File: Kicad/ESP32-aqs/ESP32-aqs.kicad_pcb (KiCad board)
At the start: 2 copper layers, 98 x 53.3 mm, 30 parts, among them J1 UART Connector, J2 JST connector SEN55, J3 ufl connector, SW1 RESET, SW2 BOOT, U1 LD1117S33TR_SOT223, U2 ESP32-WROOM-32-N8, U3 SGP41-D-R4, U4 DL-RFM95-868M

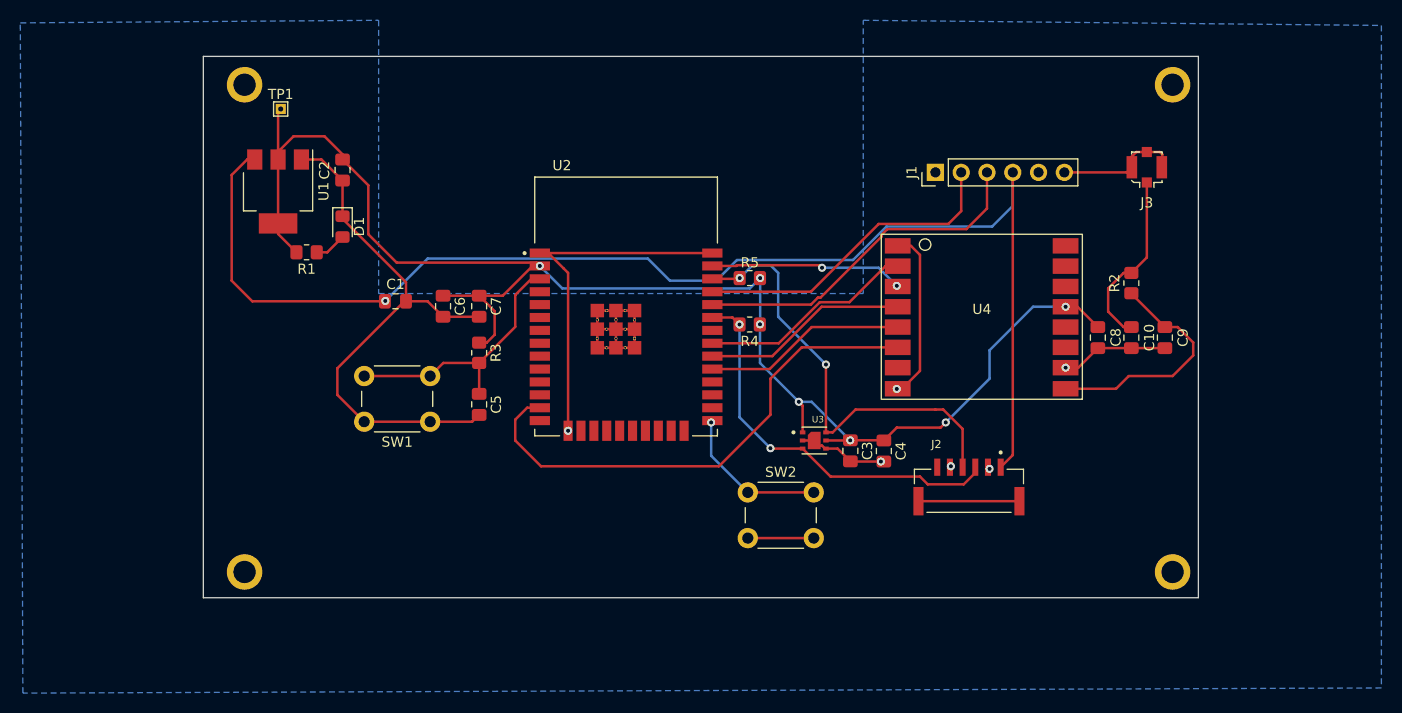
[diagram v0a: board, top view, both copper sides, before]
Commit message: PCB design geupdate
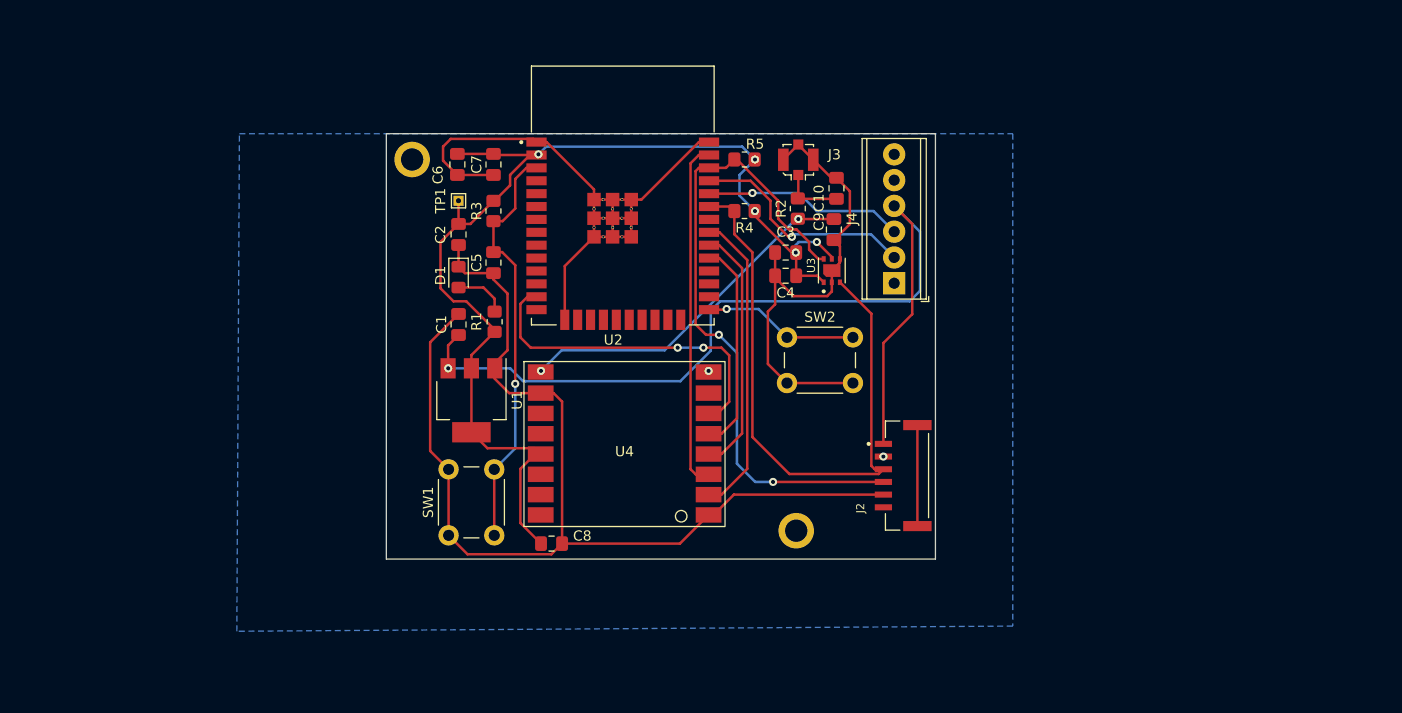
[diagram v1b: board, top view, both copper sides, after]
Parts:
- removed H1, H3: MountingHole, MountingHole:MountingHole_2.2mm_M2_ISO7380_Pad
- removed J1: UART Connector, Connector_PinHeader_2.54mm:PinHeader_1x06_P2.54mm_Vertical
- added J4: UART Connector, TerminalBlock_Phoenix:TerminalBlock_Phoenix_MPT-0,5-6-2.54_1x06_P2.54mm_Horizontal, F.Cu at (183.4, 80.8)
- SW1: value RESET -> TC-1102-B-C-B; footprint Button_Switch_THT:SW_PUSH_6mm_H7.3mm -> Button_Switch_THT:SW_PUSH_6mm
- SW2: value BOOT -> TC-1102-B-C-B; footprint Button_Switch_THT:SW_PUSH_6mm_H7.3mm -> Button_Switch_THT:SW_PUSH_6mm
- U2: value ESP32-WROOM-32-N8 -> ESP32-WROOM-32
- U4: value DL-RFM95-868M -> SX1276S8S+T-X1
- moved C8 57.5 mm to (149.6, 106.4), turned to 0 degrees
- moved H2 37.3 mm to (173.7, 105.2)
- moved U4 37.2 mm to (156.6, 95.6), turned to 0 degrees
- moved J3 34.3 mm to (173.9, 68.6)
- moved C9 34.3 mm to (177.4, 75.5)
- moved R2 33.7 mm to (173.9, 73.4)
- moved C10 32.6 mm to (177.7, 71.4), turned to -90 degrees
- moved U1 28.0 mm to (141.7, 92.3)
- moved C3 20.5 mm to (172.7, 77.7), turned to 180 degrees
- moved C4 19.8 mm to (172.7, 80.0), turned to 180 degrees
- moved R1 19.7 mm to (144.0, 84.6), turned to -90 degrees
- moved TP1 19.7 mm to (140.5, 72.6)
- moved H4 18.1 mm to (135.9, 68.6)
- moved U3 16.8 mm to (177.2, 79.5), turned to 90 degrees
- moved SW2 15.8 mm to (172.8, 86.1)
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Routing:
- net GND: track 167.5 -> 223.0 mm, vias 6 -> 2
- net +3V3: track 149.1 -> 110.5 mm, vias 7 -> 5
- net VIN: track 129.7 -> 91.5 mm
- net SDA: track 39.1 -> 61.0 mm, vias 2 -> 0
- net SCL: track 44.0 -> 65.1 mm
- net RST: track 50.6 -> 33.6 mm, vias 0 -> 2
- net MOSI: track 19.0 -> 34.3 mm, vias 2 -> 0
- net EN: track 26.2 -> 41.3 mm, vias 0 -> 1
- net TX: track 34.6 -> 19.8 mm, vias 0 -> 1
- net ANT: track 23.3 -> 35.1 mm, vias 0 -> 2
- net Net-(J3-In): track 17.7 -> 6.16 mm
- net RX: track 31.6 -> 22.6 mm, vias 0 -> 1
- net MISO: track 21.4 -> 30.3 mm
- net SCK: track 20.3 -> 24.6 mm
- net Net-(D1-A): track 3.16 -> 5.28 mm
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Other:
- board size 98 x 53.3 mm -> 54.1 x 41.9 mm
